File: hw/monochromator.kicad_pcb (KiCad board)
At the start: 2 copper layers, 100 x 45 mm, 45 parts, among them J1 USB_B, J2 UART_01X03, J3 IDC_02X03, J4 SWD_01X04, J5 Power_Terminal, J6 Screw_Terminal, SW1 SW_Push, U1 USBLC6-2SC6, U2 STM32F072CBTx, U3 CP2102, U4 MCP16301H

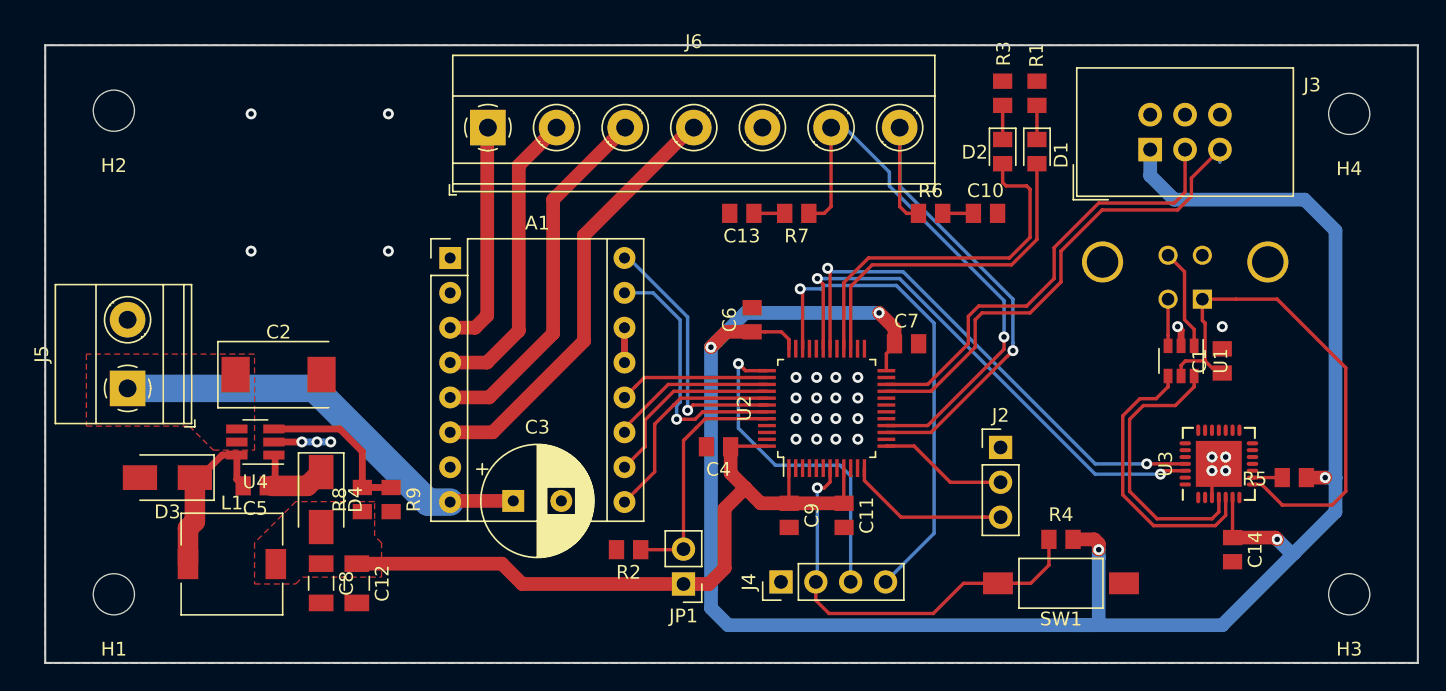
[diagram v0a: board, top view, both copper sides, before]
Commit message: Python App + GERBERS
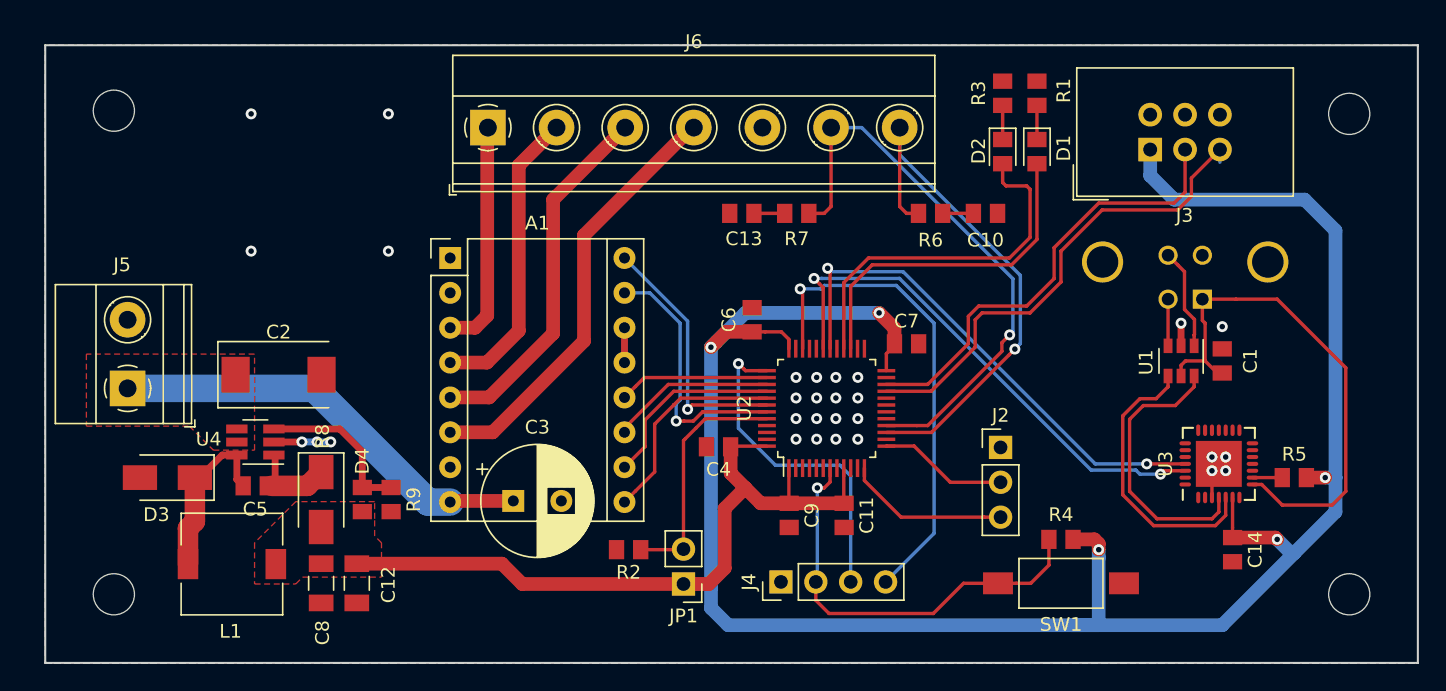
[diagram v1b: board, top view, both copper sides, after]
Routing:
- net /END_STOP2: track 40.4 -> 41.7 mm
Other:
- net class Default: clearance 0.1 -> 0.2
- rule trace_clearance: 0.1 -> 0.2
